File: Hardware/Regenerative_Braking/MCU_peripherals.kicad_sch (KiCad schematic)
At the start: 1 part, among them U1 NUCLEO-F446RE

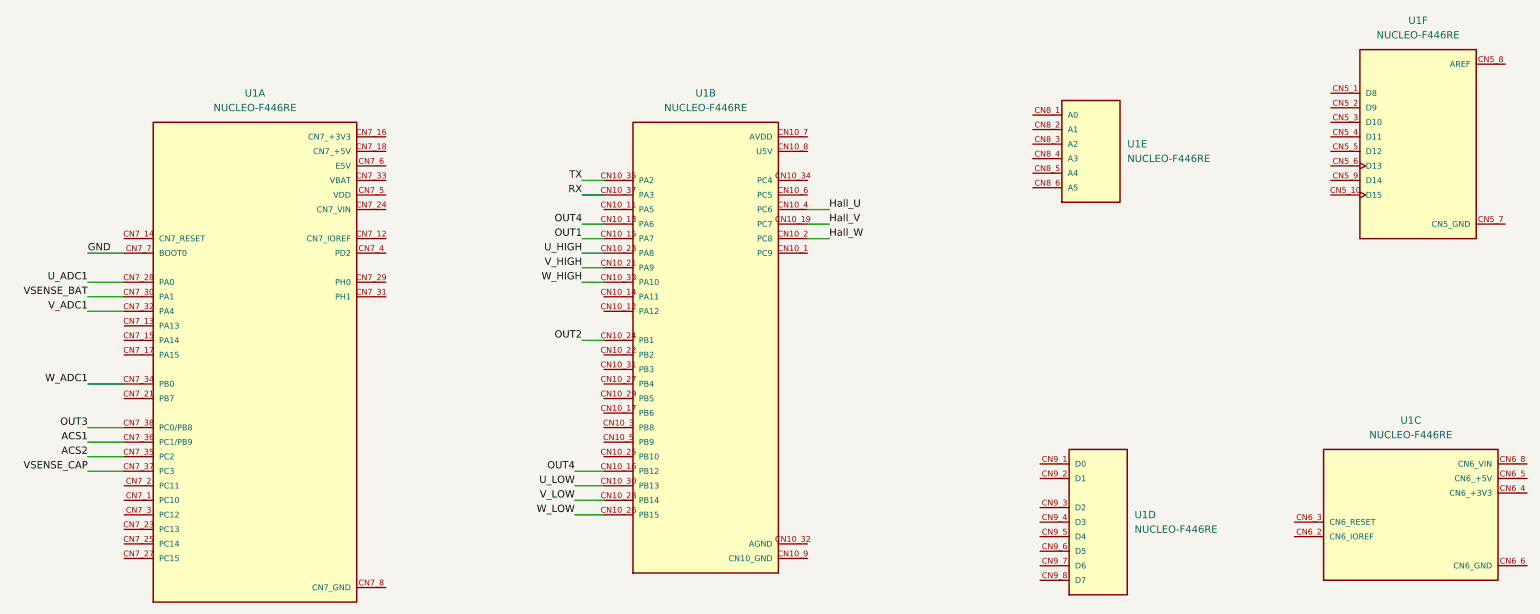
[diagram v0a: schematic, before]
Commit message: finished placement
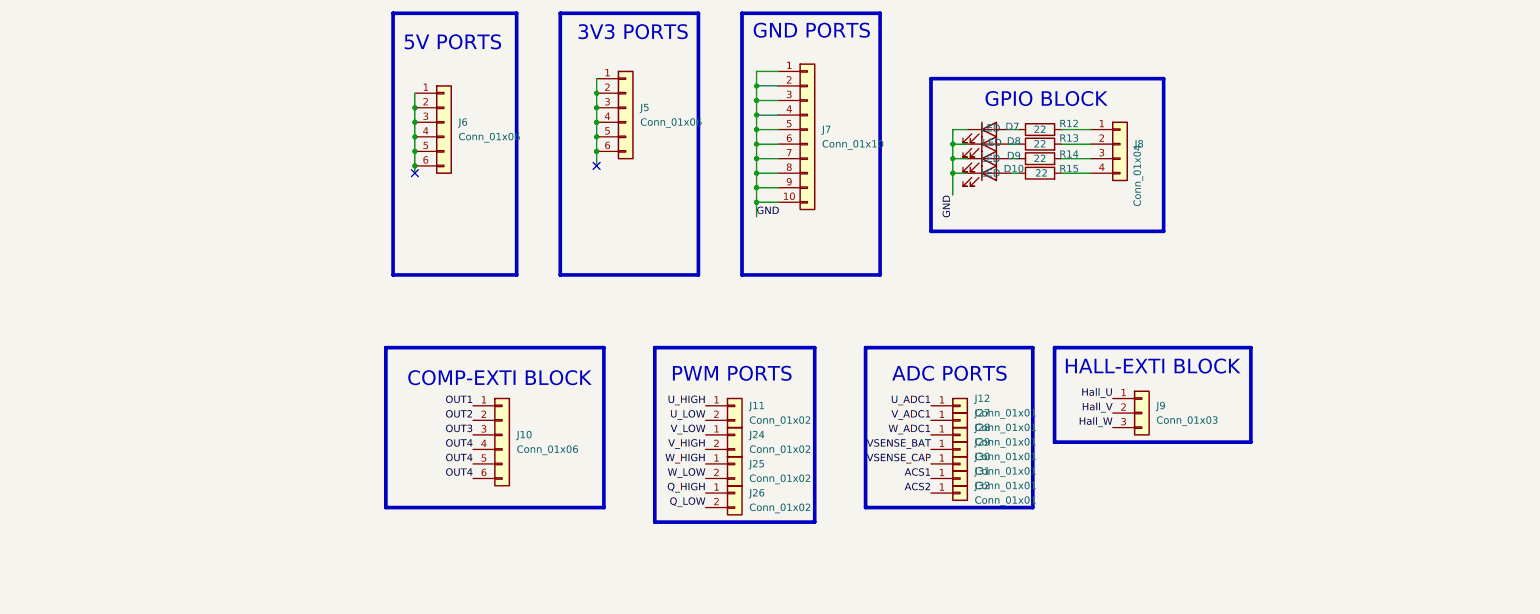
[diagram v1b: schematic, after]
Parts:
- removed U1: NUCLEO-F446RE, Regen_braking:MODULE_NUCLEO-F446RE, symbol Regen_braking:NUCLEO-F446RE
- added D10, D7, D8, D9: LED, LED_THT:LED_D5.0mm, symbol Device:LED
- added J10, J5, J6: Conn_01x06, Connector_PinHeader_2.54mm:PinHeader_1x06_P2.54mm_Vertical, symbol Connector_Generic:Conn_01x06
- added J11, J24, J25, J26: Conn_01x02, Connector_PinHeader_2.54mm:PinHeader_1x02_P2.54mm_Vertical, symbol Connector_Generic:Conn_01x02
- added J12, J27, J28, J29, J30, J31, J32: Conn_01x01, Connector_PinHeader_2.54mm:PinHeader_1x01_P2.54mm_Vertical, symbol Connector_Generic:Conn_01x01
- added J7: Conn_01x10, Connector_PinHeader_2.54mm:PinHeader_1x10_P2.54mm_Vertical, symbol Connector_Generic:Conn_01x10
- added J8: Conn_01x04, Connector_PinHeader_2.54mm:PinHeader_1x04_P2.54mm_Vertical, symbol Connector_Generic:Conn_01x04
- added J9: Conn_01x03, Connector_PinHeader_2.54mm:PinHeader_1x03_P2.54mm_Vertical, symbol Connector_Generic:Conn_01x03
- added R12, R13, R14, R15: 22, Resistor_THT:R_Axial_DIN0204_L3.6mm_D1.6mm_P7.62mm_Horizontal, symbol Device:R
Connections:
- net ACS1: now also J31.1 (Pin_1)
- net ACS2: now also J32.1 (Pin_1)
- net GND: now also D10.1 (K), D7.1 (K), D8.1 (K), D9.1 (K), J7.1 (Pin_1), J7.10 (Pin_10), J7.2 (Pin_2), J7.3 (Pin_3), J7.4 (Pin_4), J7.5 (Pin_5), J7.6 (Pin_6), J7.7 (Pin_7), J7.8 (Pin_8), J7.9 (Pin_9)
- net Hall_U: now also J9.1 (Pin_1)
- net Hall_V: now also J9.2 (Pin_2)
- net Hall_W: now also J9.3 (Pin_3)
- net OUT1: now also J10.1 (Pin_1)
- net OUT2: now also J10.2 (Pin_2)
- net OUT3: now also J10.3 (Pin_3)
- net OUT4: now also J10.4 (Pin_4), J10.5 (Pin_5), J10.6 (Pin_6)
- net U_ADC1: now also J12.1 (Pin_1)
- net U_HIGH: now also J11.1 (Pin_1)
- net U_LOW: now also J11.2 (Pin_2)
- net VSENSE_BAT: now also J29.1 (Pin_1)
- net VSENSE_CAP: now also J30.1 (Pin_1)
- net V_ADC1: now also J27.1 (Pin_1)
- net V_HIGH: now also J24.2 (Pin_2)
- net V_LOW: now also J24.1 (Pin_1)
- net W_ADC1: now also J28.1 (Pin_1)
- net W_HIGH: now also J25.1 (Pin_1)
- net W_LOW: now also J25.2 (Pin_2)
- new net: D9.2 (A), R14.1
- new net: J8.3 (Pin_3), R14.2
- new net: J6.1 (Pin_1), J6.2 (Pin_2), J6.3 (Pin_3), J6.4 (Pin_4), J6.5 (Pin_5), J6.6 (Pin_6)
- new net: J8.1 (Pin_1), R12.2
- new net: J8.2 (Pin_2), R13.2
- new net: J8.4 (Pin_4), R15.2
- new net: D8.2 (A), R13.1
- new net: D7.2 (A), R12.1
- new net: J5.1 (Pin_1), J5.2 (Pin_2), J5.3 (Pin_3), J5.4 (Pin_4), J5.5 (Pin_5), J5.6 (Pin_6)
- new net: D10.2 (A), R15.1
- new net Q_HIGH: J26.1 (Pin_1)
- new net Q_LOW: J26.2 (Pin_2)
- no-connect marks 0 -> 2
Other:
- note added: "3V3 PORTS"
- note added: "5V PORTS"
- note added: "ADC PORTS"
- note added: "COMP-EXTI BLOCK"
- note added: "GND PORTS"
- note added: "GPIO BLOCK"
- note added: "HALL-EXTI BLOCK"
- note added: "PWM PORTS"
